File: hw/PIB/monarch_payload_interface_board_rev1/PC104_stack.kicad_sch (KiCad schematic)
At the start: 1 part, among them U1 Payload

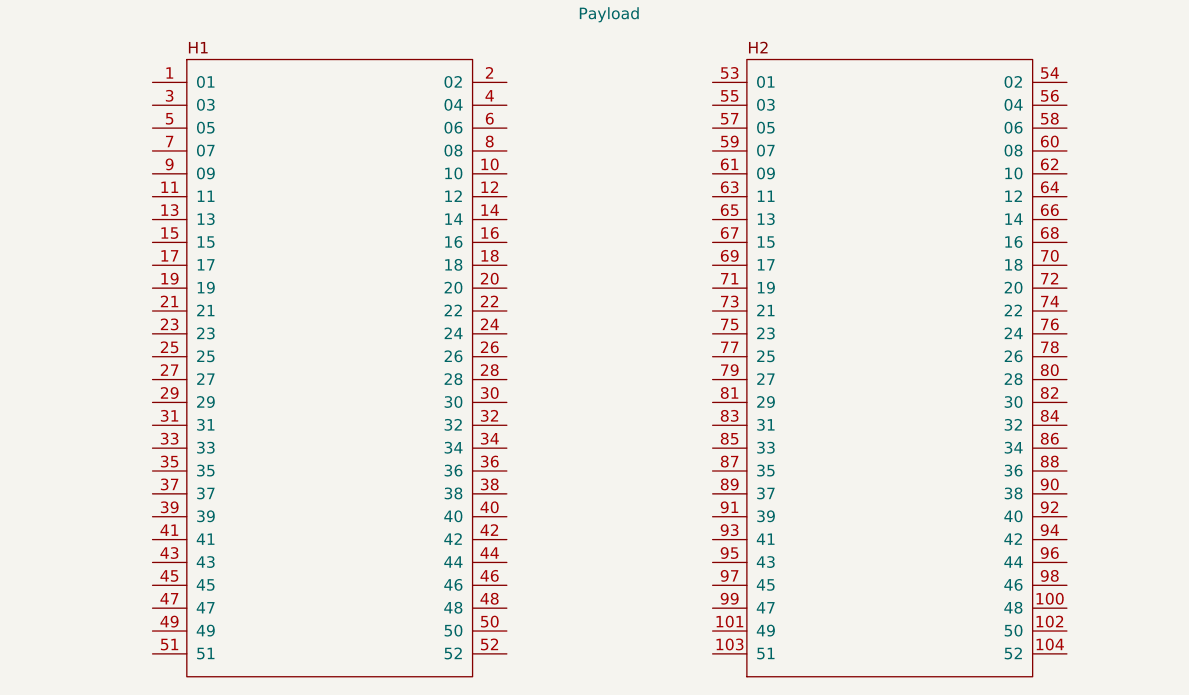
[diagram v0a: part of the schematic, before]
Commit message: More components
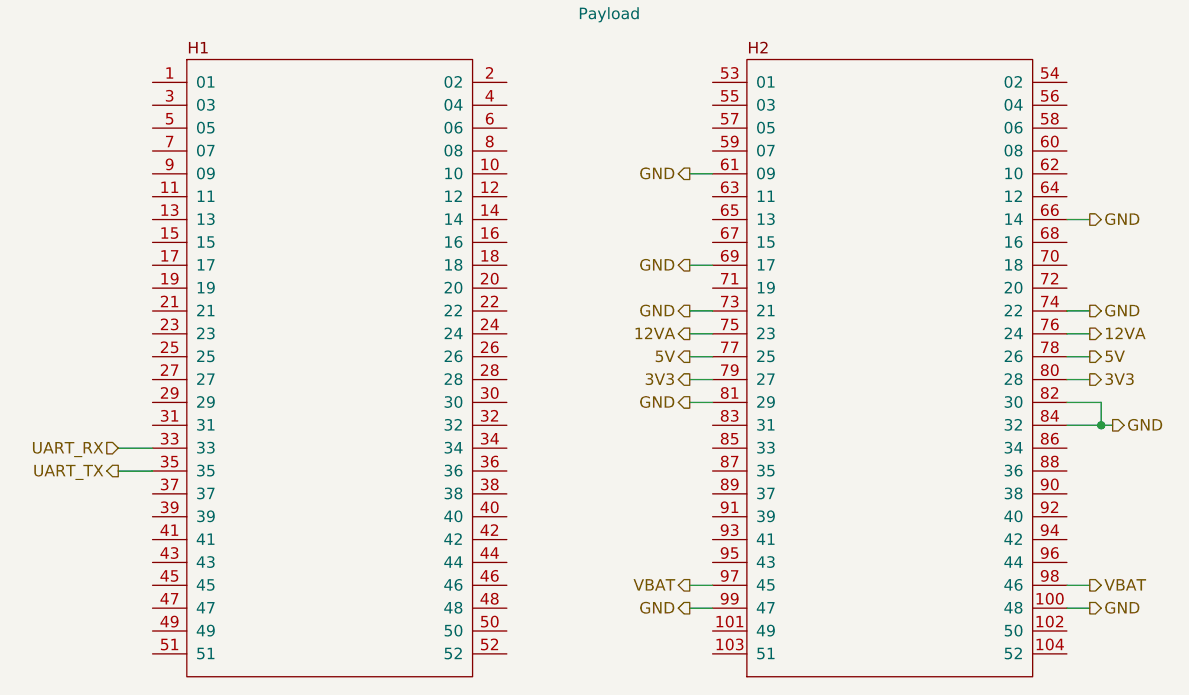
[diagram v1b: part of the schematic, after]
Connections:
- net GND: now reaches U1.100 (48)
- net GND: now also U1.61 (09), U1.66 (14), U1.69 (17), U1.73 (21), U1.74 (22), U1.81 (29), U1.82 (30), U1.84 (32), U1.99 (47)
- net UART_RX: now reaches U1.33
- net UART_TX: now reaches U1.35
- net 12VA: now reaches U1.75 (23)
- net 12VA: now also U1.76 (24)
- net 5V: now reaches U1.77 (25)
- net 5V: now also U1.78 (26)
- net 3V3: now reaches U1.79 (27)
- net 3V3: now also U1.80 (28)
- net VBAT: now reaches U1.97 (45)
- net VBAT: now also U1.98 (46)

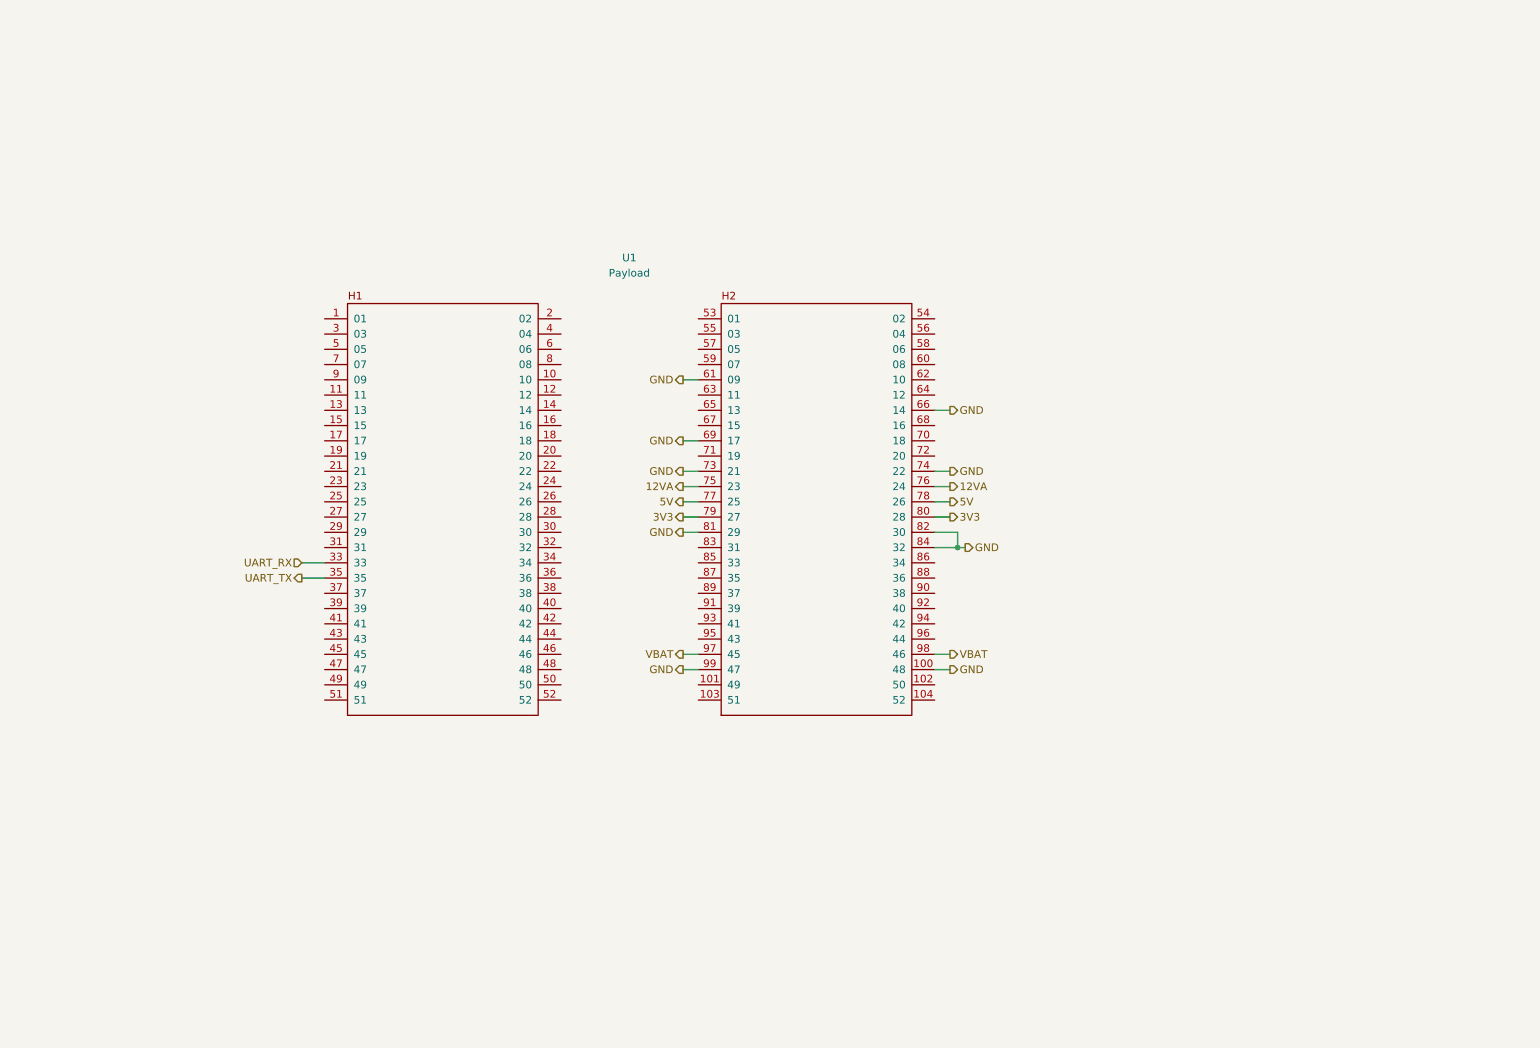
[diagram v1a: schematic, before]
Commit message: PCB updates
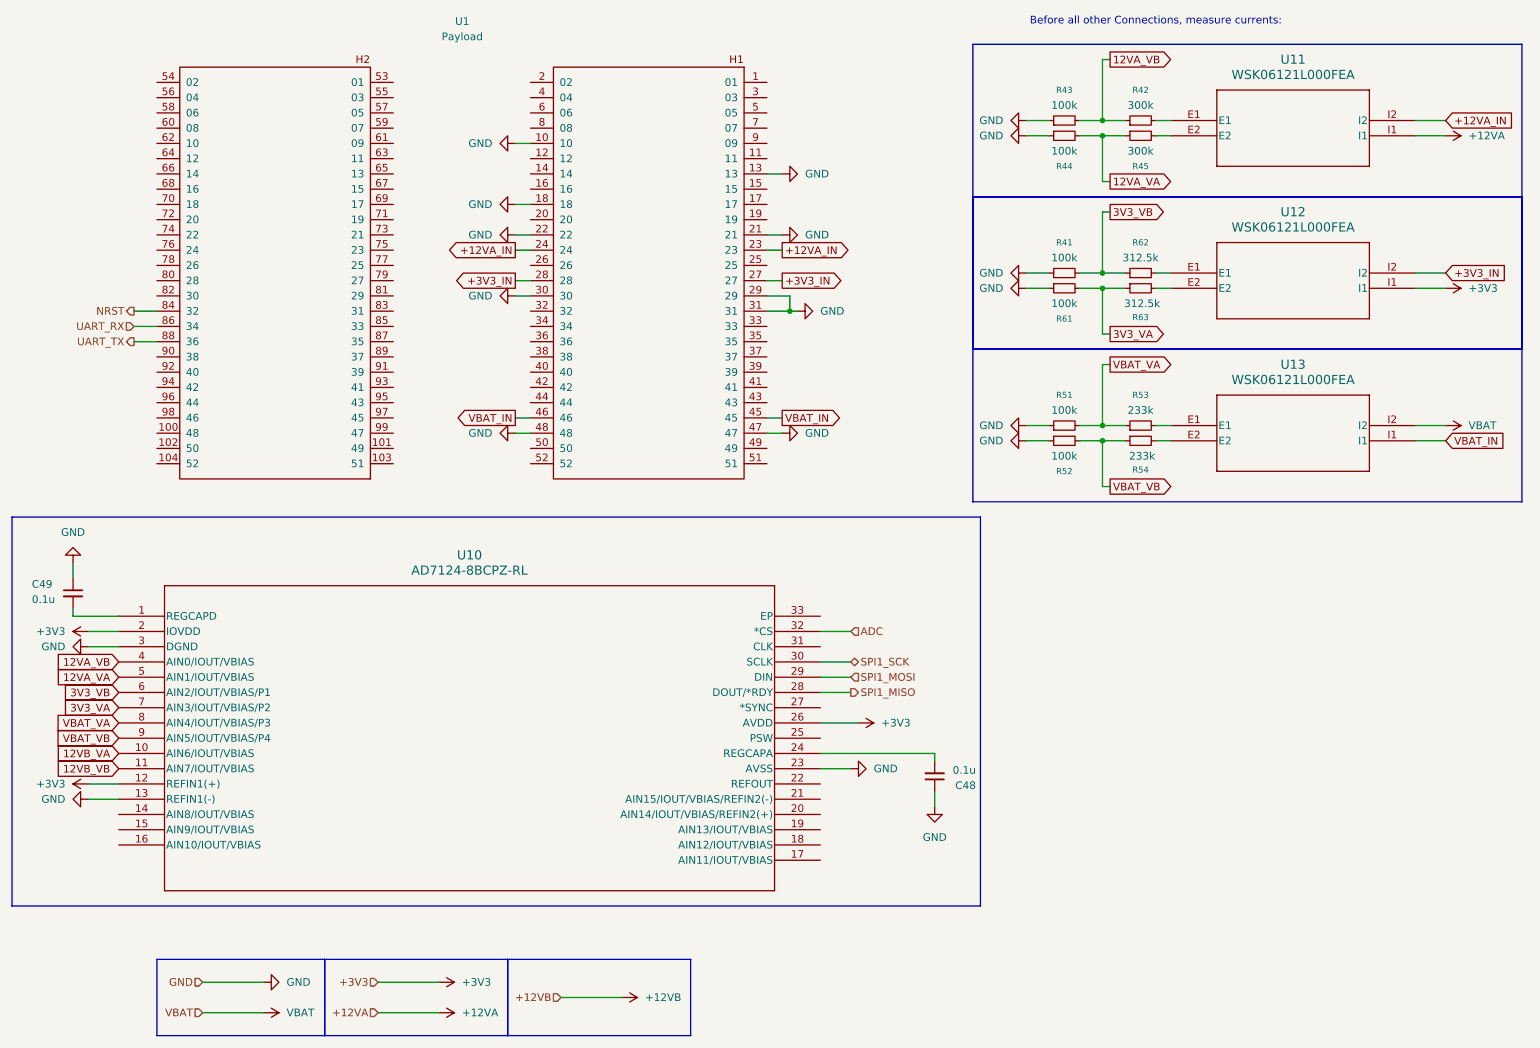
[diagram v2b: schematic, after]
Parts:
- added C48, C49: 0.1u, Capacitor_SMD:C_0603_1608Metric, symbol Device:C_Small
- added R41, R43, R44, R51, R52, R61: 100k, Resistor_SMD:R_0603_1608Metric, symbol Device:R_Small
- added R42, R45: 300k, Resistor_SMD:R_0603_1608Metric, symbol Device:R_Small
- added R53, R54: 233k, Resistor_SMD:R_0603_1608Metric, symbol Device:R_Small
- added R62, R63: 312.5k, Resistor_SMD:R_0603_1608Metric, symbol Device:R_Small
- added U10: AD7124-8BCPZ-RL, AD7124:CP-32-12_ADI-L, symbol AD7124:AD7124-8BCPZ-RL
- added U11, U12, U13: WSK06121L000FEA, WSK:SMT_121L000FEA_VIS, symbol WSK:WSK06121L000FEA
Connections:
- net GND: now also U1.10, U1.13, U1.18, U1.21, U1.22, U1.29, U1.30, U1.31, U1.47, U1.48, C48.1, C49.1, R41.1, R43.1, R44.1, R51.1, R52.1, R61.1, U10.13 (REFIN1(-)), U10.23 (AVSS), U10.3 (DGND); no longer U1.100 (48), U1.61 (09), U1.66 (14), U1.69 (17), U1.73 (21), U1.74 (22), U1.81 (29), U1.82 (30), U1.84 (32), U1.99 (47)
- net UART_RX: now also U1.86 (34); no longer U1.33
- net UART_TX: now also U1.88 (36); no longer U1.35
- net VBAT: now also U13.I2; no longer U1.97 (45), U1.98 (46)
- net +12VA_IN: now reaches U1.23
- net +12VA_IN: now also U1.24, U11.I2
- net +3V3_IN: now reaches U1.27
- net +3V3_IN: now also U1.28, U12.I2
- net VBAT_IN: now reaches U1.45
- net VBAT_IN: now also U1.46, U13.I1
- net 12VA: no longer names the net of U1.75 (23)
- net 12VA: no longer U1.76 (24)
- net 3V3: no longer names the net of U1.79 (27)
- net 3V3: no longer U1.80 (28)
- net 5V: no longer names the net of U1.77 (25)
- net 5V: no longer U1.78 (26)
- new net: R62.2, U12.E1
- new net: R42.2, U11.E1
- new net: R45.2, U11.E2
- new net: C48.2, U10.24 (REGCAPA)
- new net: R63.2, U12.E2
- new net: R53.2, U13.E1
- new net: C49.2, U10.1 (REGCAPD)
- new net: R54.2, U13.E2
- new net +12VA: U11.I1
- new net +3V3: U10.12 (REFIN1(+)), U10.2 (IOVDD), U10.26 (AVDD), U12.I1
- new net 12VA_VA: R44.2, R45.1, U10.5 (AIN1/IOUT/VBIAS)
- new net 12VA_VB: R42.1, R43.2, U10.4 (AIN0/IOUT/VBIAS)
- new net 12VB_VA: U10.10 (AIN6/IOUT/VBIAS)
- new net 12VB_VB: U10.11 (AIN7/IOUT/VBIAS)
- new net 3V3_VA: R61.2, R63.1, U10.7 (AIN3/IOUT/VBIAS/P2)
- new net 3V3_VB: R41.2, R62.1, U10.6 (AIN2/IOUT/VBIAS/P1)
- new net ADC: U10.32 (*CS)
- new net NRST: U1.84 (32)
- new net SPI1_MISO: U10.28 (DOUT/*RDY)
- new net SPI1_MOSI: U10.29 (DIN)
- new net SPI1_SCK: U10.30 (SCLK)
- new net VBAT_VA: R51.2, R53.1, U10.8 (AIN4/IOUT/VBIAS/P3)
- new net VBAT_VB: R52.2, R54.1, U10.9 (AIN5/IOUT/VBIAS/P4)
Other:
- note added: "Before all other Connections, measure currents:"
- moved on the sheet: U1
